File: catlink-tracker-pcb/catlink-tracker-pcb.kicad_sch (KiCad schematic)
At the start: 33 parts, among them J1 S2B-PH-K, J2 U.FL, U1 STM32L412K8Tx, U2 TLV75530PDBV, U3 Ai-Thinker-Ra-01S, U4 E108-GN03

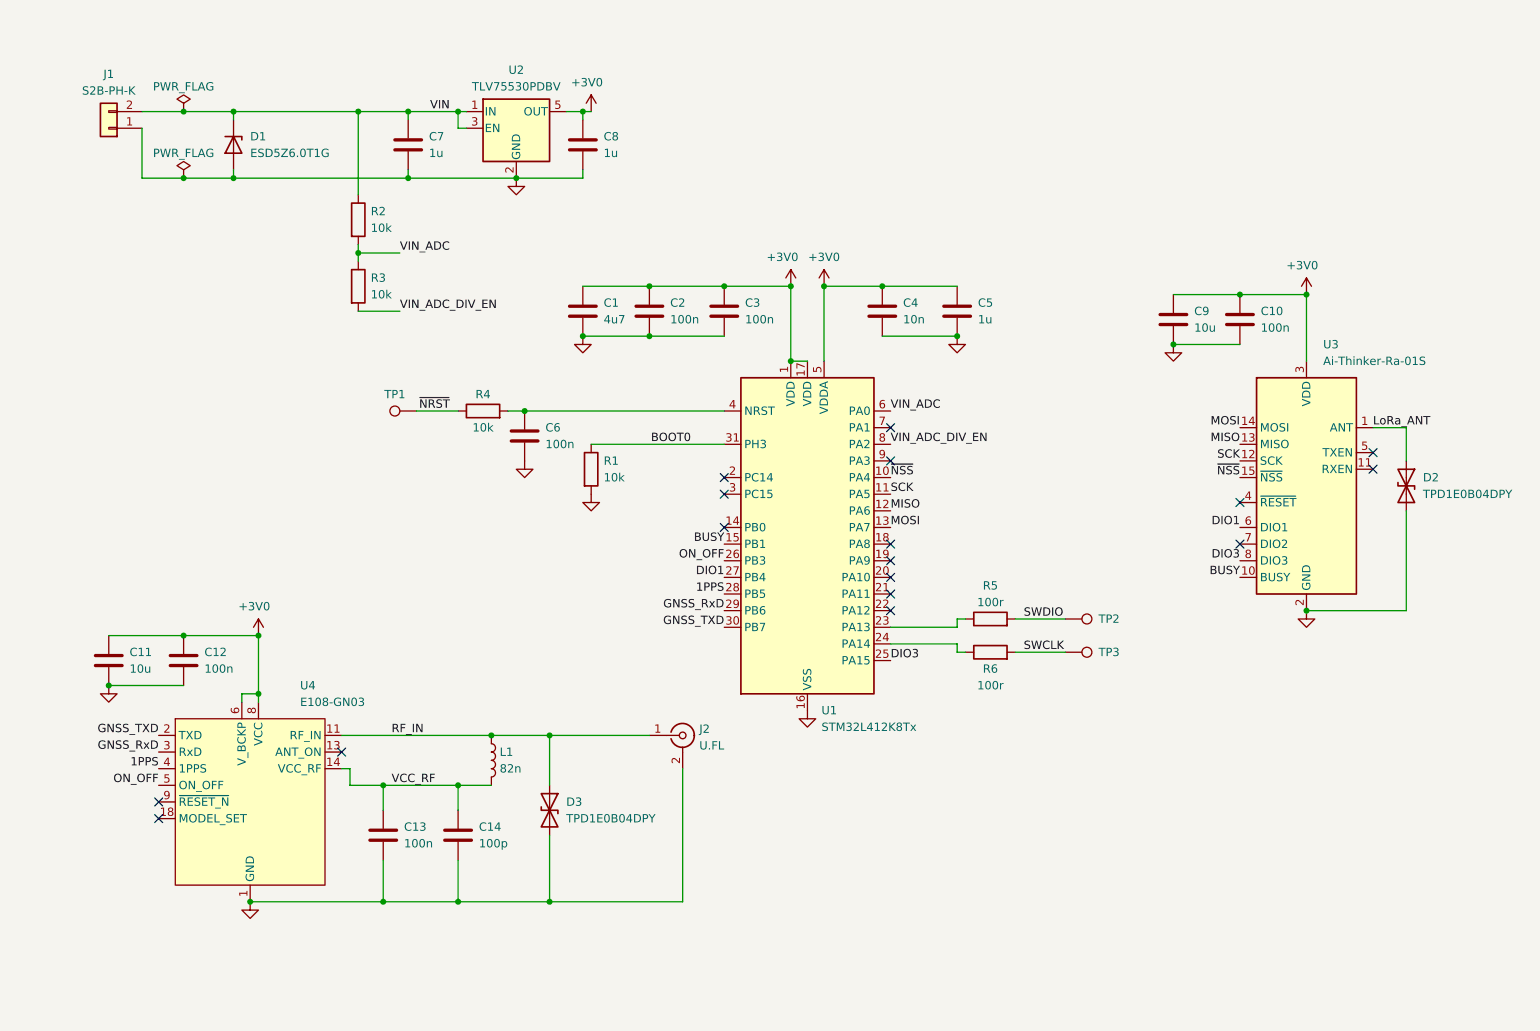
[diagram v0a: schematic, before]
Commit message: v0.1
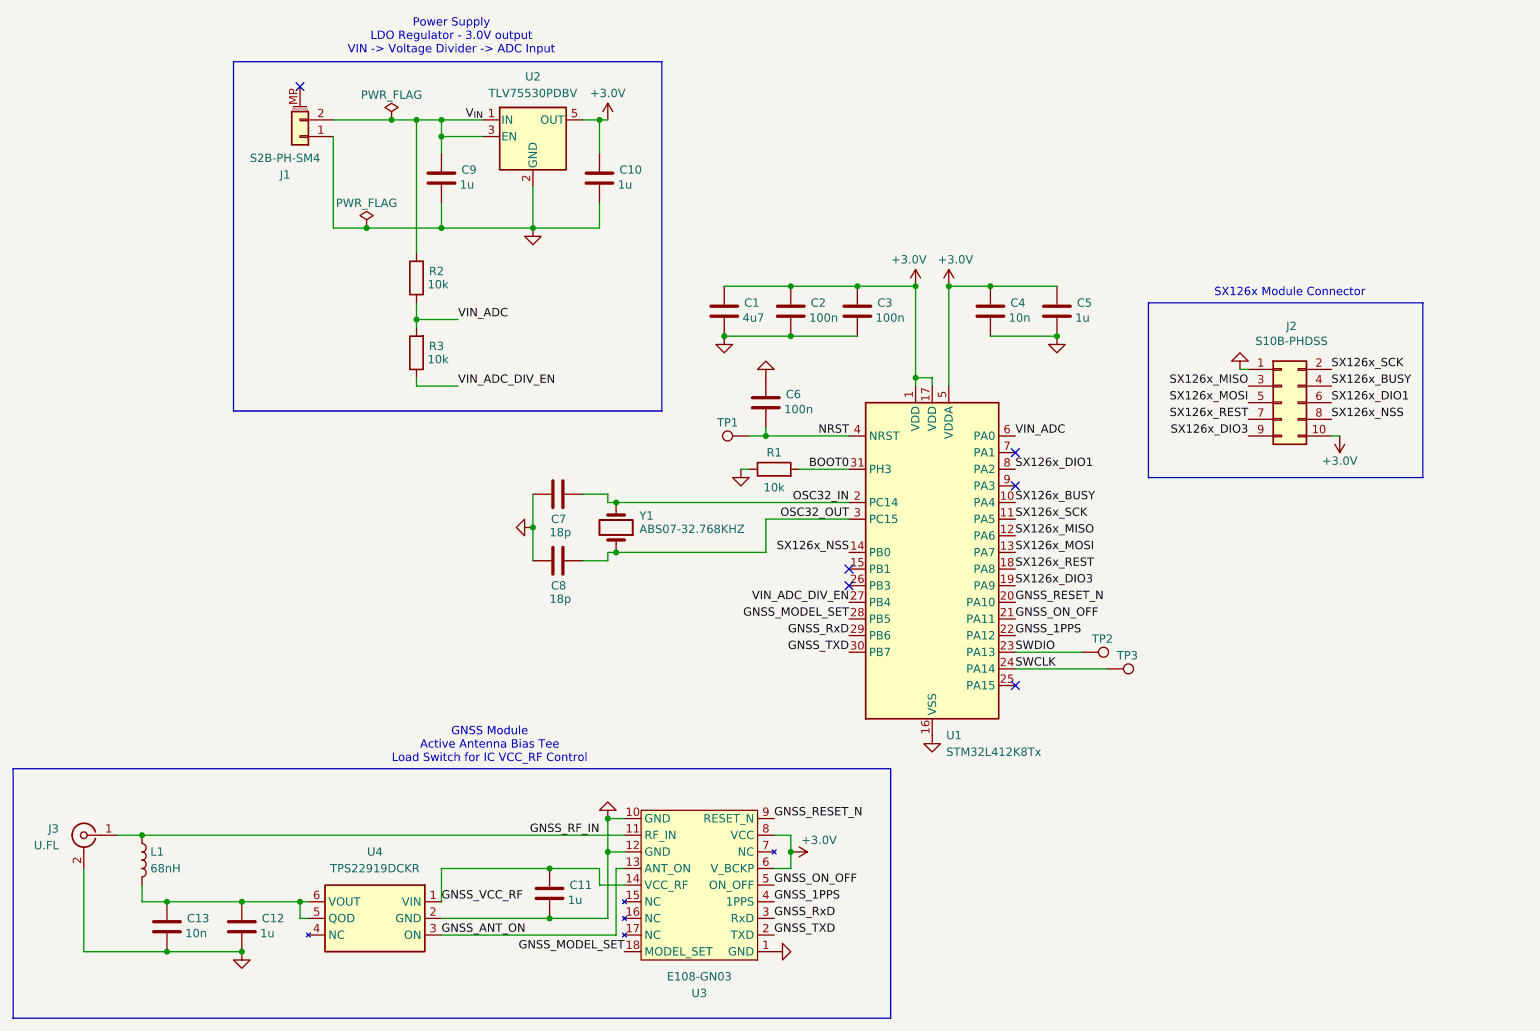
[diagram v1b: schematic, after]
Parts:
- removed C14: 100p, Custom:C_0603_1608Metric, symbol Device:C
- removed D1: ESD5Z6.0T1G, Custom:D_SOD-523, symbol Device:D_Zener
- removed D2, D3: TPD1E0B04DPY, Custom:D_Texas_DPY0002A_0.6x1mm_P0.65mm, symbol Device:D_TVS
- removed J1: S2B-PH-K, Connector_JST:JST_PH_S2B-PH-K_1x02_P2.00mm_Horizontal, symbol Connector_Generic:Conn_01x02
- removed J2: U.FL, Connector_Coaxial:U.FL_Hirose_U.FL-R-SMT-1_Vertical, symbol Connector:Conn_Coaxial
- removed R4: 10k, Custom:R_0603_1608Metric, symbol Device:R
- removed R5, R6: 100r, Custom:R_0603_1608Metric, symbol Device:R
- removed U3: Ai-Thinker-Ra-01S, Custom:Ai-Thinker-Ra-01S, symbol Custom:Ai-Thinker-Ra-01S
- removed U4: E108-GN03, Custom:E108-GN03, symbol Custom:E108-GN03
- added J1: S2B-PH-SM4, Connector_JST:JST_PH_S2B-PH-SM4-TB_1x02-1MP_P2.00mm_Horizontal, symbol Connector_Generic_MountingPin:Conn_01x02_MountingPin
- added J2: S10B-PHDSS, Connector_JST:JST_PHD_S10B-PHDSS_2x05_P2.00mm_Horizontal, symbol Connector_Generic:Conn_02x05_Odd_Even
- added J3: U.FL, Connector_Coaxial:U.FL_Hirose_U.FL-R-SMT-1_Vertical, symbol Connector:Conn_Coaxial
- added U3: E108-GN03, Custom:E108-GN03, symbol Custom:E108-GN03
- added U4: TPS22919DCKR, Package_TO_SOT_SMD:SOT-363_SC-70-6, symbol Custom:TPS22919DCKR
- added Y1: ABS07-32.768KHZ, Crystal:Crystal_SMD_3215-2Pin_3.2x1.5mm, symbol Device:Crystal
- C1, C2, C3, C4, C5, C6: footprint Custom:C_0603_1608Metric -> Capacitor_SMD:C_0603_1608Metric
- C10, C12: value 100n -> 1u; footprint Custom:C_0603_1608Metric -> Capacitor_SMD:C_0603_1608Metric
- C11, C9: value 10u -> 1u; footprint Custom:C_0805_2012Metric -> Capacitor_SMD:C_0603_1608Metric
- C13: value 100n -> 10n; footprint Custom:C_0603_1608Metric -> Capacitor_SMD:C_0603_1608Metric
- C7, C8: value 1u -> 18p; footprint Custom:C_0603_1608Metric -> Capacitor_SMD:C_0603_1608Metric
- L1: value 82n -> 68nH; footprint Custom:L_0603_1608Metric -> Inductor_SMD:L_0603_1608Metric
- R1, R2, R3: footprint Custom:R_0603_1608Metric -> Resistor_SMD:R_0603_1608Metric
- TP1, TP2, TP3: value TestPoint -> ~; footprint Custom:TestPoint_THT_D1.4mm_Drill0.8mm -> Custom:TestPoint
- U1: footprint Custom:LQFP-32_7x7mm_P0.8mm -> Package_QFP:LQFP-32_7x7mm_P0.8mm
- U2: footprint Custom:SOT-23-5 -> Package_TO_SOT_SMD:SOT-23-5
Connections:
- net DIO1 is gone; now on net VIN_ADC_DIV_EN: U1.27 (PB4)
- net ~{NRST} is gone; now on net NRST: TP1.1
- net BOOT0: now also R1.2; no longer R1.1
- net GND: now also C6.1, C7.1, C8.1, R1.1, J1.1 (Pin_1), J2.1 (Pin_1), J3.2 (Ext), U3.1 (GND), U3.10 (GND), U3.12 (GND), U4.2 (GND); no longer C6.2, C7.2, C8.2, R1.2
- net GNSS_RxD: now also U3.3 (RxD)
- net GNSS_TXD: now also U3.2 (TXD)
- net SWCLK: now also U1.24 (PA14)
- net SWDIO: now also U1.23 (PA13)
- net VIN_ADC: now also R2.1, R3.2; no longer R2.2, R3.1
- net VIN_ADC_DIV_EN: now also R3.1; no longer R3.2, U1.8 (PA2)
- net NRST: now reaches U1.4 (NRST)
- net NRST: now also C6.2; no longer C6.1
- net SX126x_NSS: now reaches U1.14 (PB0)
- net SX126x_NSS: now also J2.8 (Pin_8)
- net SX126x_REST: now reaches U1.18 (PA8)
- net SX126x_REST: now also J2.7 (Pin_7)
- net SX126x_DIO3: now reaches U1.19 (PA9)
- net SX126x_DIO3: now also J2.9 (Pin_9)
- net OSC32_IN: now reaches U1.2 (PC14)
- net OSC32_IN: now also C7.2, Y1.2
- net GNSS_RESET_N: now reaches U1.20 (PA10)
- net GNSS_RESET_N: now also U3.9 (RESET_N)
- net GNSS_ON_OFF: now reaches U1.21 (PA11)
- net GNSS_ON_OFF: now also U3.5 (ON_OFF)
- net GNSS_1PPS: now reaches U1.22 (PA12)
- net GNSS_1PPS: now also U3.4 (1PPS)
- net OSC32_OUT: now reaches U1.3 (PC15)
- net OSC32_OUT: now also C8.2, Y1.1
- net +3V0 renamed +3.0V
- net +3.0V: now also J2.10 (Pin_10), U3.6 (V_BCKP), U3.8 (VCC); no longer C11.1, C12.1, C8.1, C9.1
- net 1PPS renamed GNSS_MODEL_SET
- net GNSS_MODEL_SET: now also U3.18 (MODEL_SET)
- net BUSY: no longer names the net of U1.15 (PB1)
- net DIO3: no longer names the net of U1.25 (PA15)
- net MISO renamed SX126x_MISO
- net SX126x_MISO: now also J2.3 (Pin_3)
- net MOSI renamed SX126x_MOSI
- net SX126x_MOSI: now also J2.5 (Pin_5)
- net ON_OFF: no longer names the net of U1.26 (PB3)
- net RF_IN renamed GNSS_RF_IN
- net GNSS_RF_IN: now also J3.1 (In), U3.11 (RF_IN)
- net SCK renamed SX126x_SCK
- net SX126x_SCK: now also J2.2 (Pin_2)
- net VCC_RF: no longer names the net of C13.1, L1.2
- net VCC_RF: now also C12.1, U4.5 (QOD), U4.6 (VOUT)
- net VIN renamed V_{IN}
- net V_{IN}: now also C9.1, R2.2, J1.2 (Pin_2); no longer C7.1, R2.1
- net ~{NSS} renamed SX126x_BUSY
- net SX126x_BUSY: now also J2.4 (Pin_4)
- new net GNSS_ANT_ON: U3.13 (ANT_ON), U4.3 (ON)
- new net GNSS_VCC_RF: C11.1, U3.14 (VCC_RF), U4.1 (VIN)
- new net SX126x_DIO1: J2.6 (Pin_6), U1.8 (PA2)
- no-connect marks 17 -> 6
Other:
- note added: "GNSS Module Active Antenna Bias Tee Load Switch for IC VCC_RF Control"
- note added: "Power Supply LDO Regulator - 3.0V output VIN -> Voltage Divider -> ADC Input"
- note added: "SX126x Module Connector"
- title: CatLink Tracker -> CatLink Development
